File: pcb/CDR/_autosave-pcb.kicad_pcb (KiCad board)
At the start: 2 copper layers, 11 parts, among them J4 Conn_01x03_Male, J5 Conn_01x04_Female, J6 Conn_01x08_Female, J7 Conn_01x02_Female, U1 ATmega328-P, Y1 16MHz

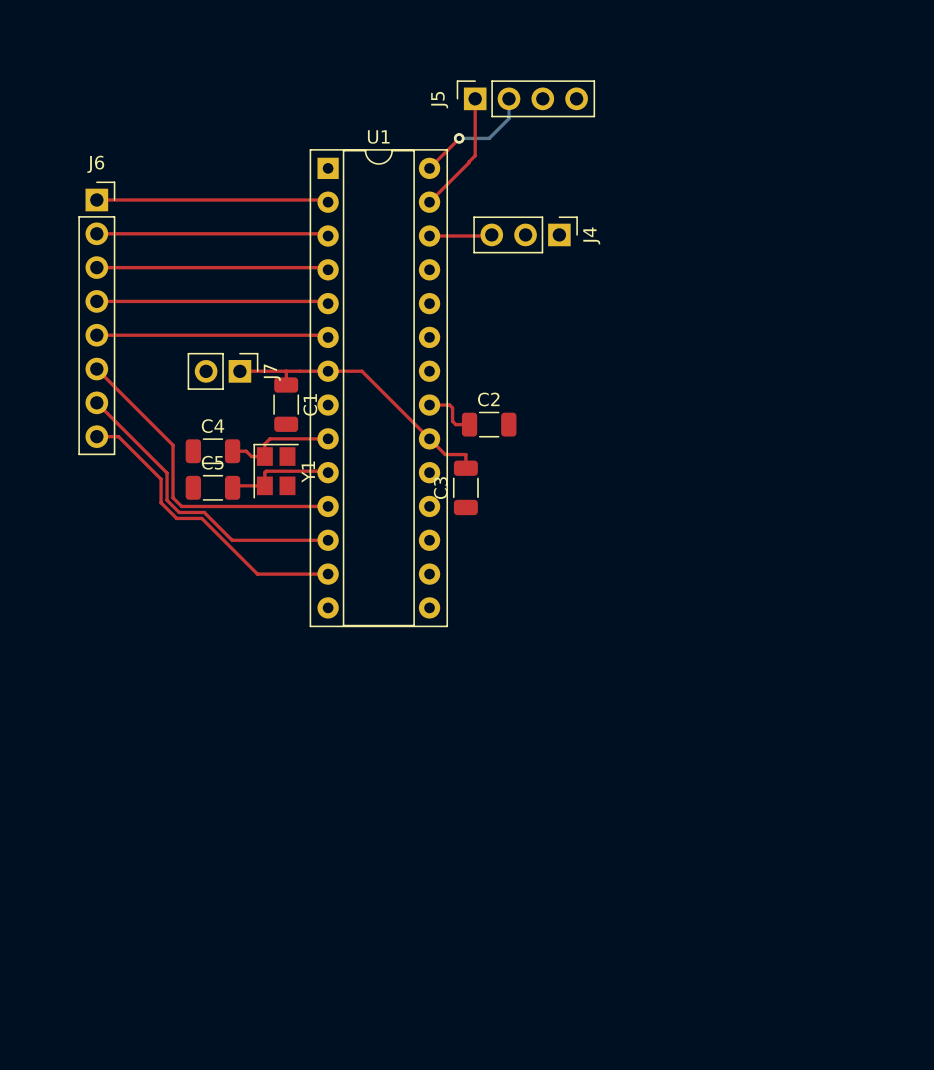
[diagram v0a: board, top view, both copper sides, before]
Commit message: cdr pcb
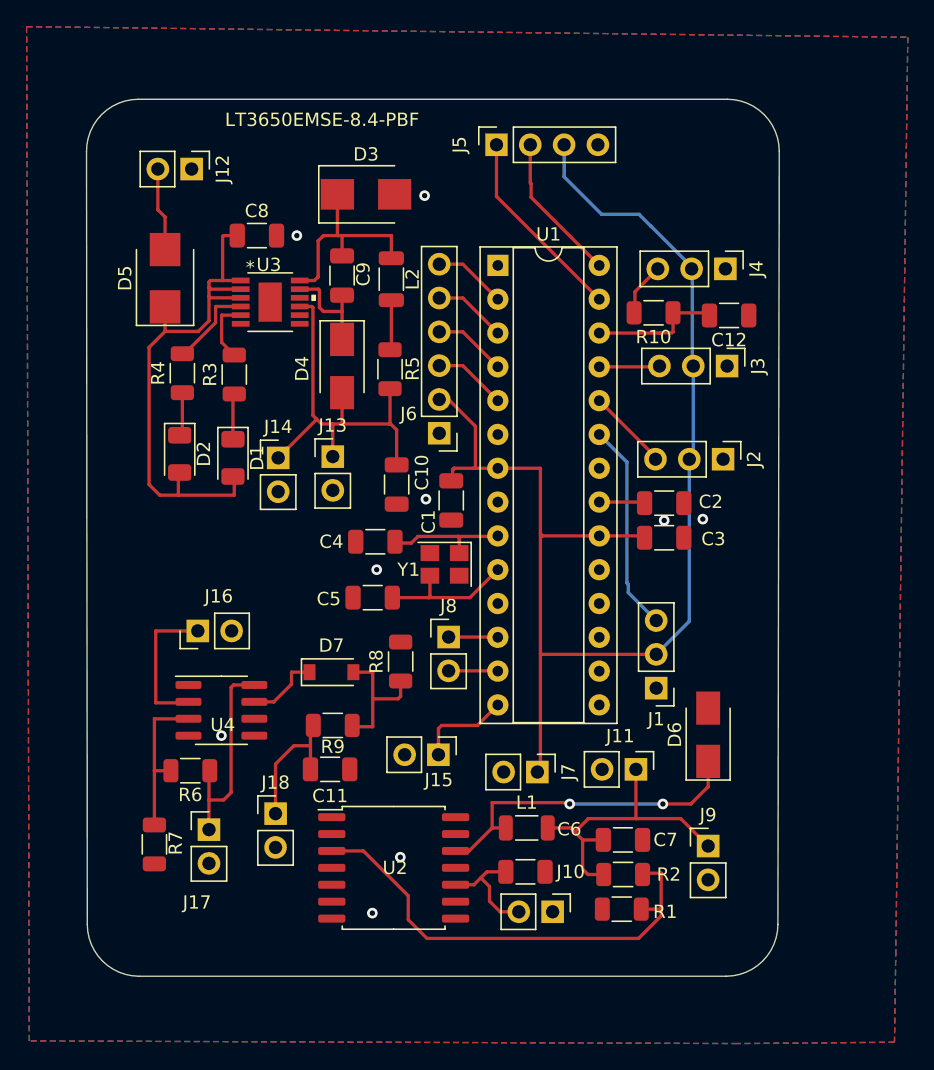
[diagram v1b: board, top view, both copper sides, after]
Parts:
- added C10: 10uF, Capacitor_SMD:C_1206_3216Metric, F.Cu at (128.3, 104.0)
- added C11: 10uF, Capacitor_SMD:C_1206_3216Metric, F.Cu at (123.3, 125.4)
- added C12: 10uF, Capacitor_SMD:C_1206_3216Metric, F.Cu at (153.3, 91.3)
- added C6: 22uF, Capacitor_SMD:C_1206_3216Metric, F.Cu at (138.0, 133.1)
- added C7: 220uF, Capacitor_SMD:C_1206_3216Metric, F.Cu at (145.3, 130.7)
- added C8: 10uF, Capacitor_SMD:C_1206_3216Metric, F.Cu at (117.8, 85.3)
- added C9: 1uF, Capacitor_SMD:C_1206_3216Metric, F.Cu at (124.2, 88.3)
- added D1: Red, Diode_SMD:D_1206_3216Metric, F.Cu at (116.0, 102.0)
- added D2: Green, Diode_SMD:D_1206_3216Metric, F.Cu at (112.0, 101.7)
- added D3: CMPSH3-40MA, Diode_SMD:D_SMB, F.Cu at (126.0, 82.2)
- added D4: CMPSH1-4, Diode_SMD:D_SMA, F.Cu at (124.2, 95.1)
- added D5: CMPSH3-40MA, Diode_SMD:D_SMB, F.Cu at (110.9, 88.5)
- added D6: 11DQ06, Diode_SMD:D_SMA, F.Cu at (151.7, 122.8)
- added D7: 1V, Diode_SMD:D_SOD-123, F.Cu at (123.4, 118.1)
- added J1: Conn_01x03_Male, Connector_PinHeader_2.54mm:PinHeader_1x03_P2.54mm_Vertical, F.Cu at (147.8, 119.3)
- added J10: V Reg in, Connector_PinHeader_2.54mm:PinHeader_1x02_P2.54mm_Vertical, F.Cu at (140.0, 136.1)
- added J11: V reg out, Connector_PinHeader_2.54mm:PinHeader_1x02_P2.54mm_Vertical, F.Cu at (146.3, 125.4)
- added J12: V Solar, Connector_PinHeader_2.54mm:PinHeader_1x02_P2.54mm_Vertical, F.Cu at (112.9, 80.3)
- added J13: V batt, Connector_PinHeader_2.54mm:PinHeader_1x02_P2.54mm_Vertical, F.Cu at (123.5, 101.9)
- added J14: V chrg out, Connector_PinHeader_2.54mm:PinHeader_1x02_P2.54mm_Vertical, F.Cu at (119.4, 102.0)
- added J15: V Low Batt in, Connector_PinHeader_2.54mm:PinHeader_1x02_P2.54mm_Vertical, F.Cu at (131.4, 124.3)
- added J16: V ref in, Connector_PinHeader_2.54mm:PinHeader_1x02_P2.54mm_Vertical, F.Cu at (113.4, 115.0)
- added J17: V Batt in, Connector_PinHeader_2.54mm:PinHeader_1x02_P2.54mm_Vertical, F.Cu at (114.2, 129.9)
- added J18: V Low Batt out, Connector_PinHeader_2.54mm:PinHeader_1x02_P2.54mm_Vertical, F.Cu at (119.2, 128.7)
- added J2: Conn_01x03_Male, Connector_PinHeader_2.54mm:PinHeader_1x03_P2.54mm_Vertical, F.Cu at (152.8, 102.1)
- added J3: Conn_01x03_Male, Connector_PinHeader_2.54mm:PinHeader_1x03_P2.54mm_Vertical, F.Cu at (153.1, 95.1)
- added J8: Cell Module, Connector_PinHeader_2.54mm:PinHeader_1x02_P2.54mm_Vertical, F.Cu at (132.2, 115.5)
- added J9: V reg out, Connector_PinHeader_2.54mm:PinHeader_1x02_P2.54mm_Vertical, F.Cu at (151.7, 131.2)
- added L1: 330 uH, Inductor_SMD:L_1206_3216Metric, F.Cu at (138.1, 129.8)
- added L2: 10uH, Inductor_SMD:L_1206_3216Metric, F.Cu at (127.9, 88.6)
- added R1: 1K, Resistor_SMD:R_1206_3216Metric, F.Cu at (145.2, 135.9)
- added R10: 0/160, Resistor_SMD:R_1206_3216Metric, F.Cu at (147.6, 91.1)
- added R2: 3.1k, Resistor_SMD:R_1206_3216Metric, F.Cu at (145.3, 133.3)
- added R3: 5.1k, Resistor_SMD:R_1206_3216Metric, F.Cu at (116.1, 95.7)
- added R4: 5.1k, Resistor_SMD:R_1206_3216Metric, F.Cu at (112.2, 95.6)
- added R5: 0.05, Resistor_SMD:R_1206_3216Metric, F.Cu at (127.8, 95.3)
- added R6: 100k, Resistor_SMD:R_1206_3216Metric, F.Cu at (112.8, 125.5)
- added R7: 220k, Resistor_SMD:R_1206_3216Metric, F.Cu at (110.1, 131.0)
- added R8: 50k, Resistor_SMD:R_1206_3216Metric, F.Cu at (128.6, 117.3)
- added R9: 160, Resistor_SMD:R_1206_3216Metric, F.Cu at (123.5, 122.1)
- added U2: LM2574HVM-12, Package_SO:SOIC-14W_7.5x9mm_P1.27mm, F.Cu at (128.1, 132.8)
- added U3: LT3650EMSE-8.4-PBF, footprints:LT3650EMSE-8.4-PBF, F.Cu at (118.8, 90.3)
- added U4: LM311, Package_SO:SOIC-8_3.9x4.9mm_P1.27mm, F.Cu at (115.1, 121.0)
- J6: value Conn_01x08_Female -> SD Card Reader; footprint Connector_PinSocket_2.54mm:PinSocket_1x08_P2.54mm_Vertical -> Connector_PinHeader_2.54mm:PinHeader_1x06_P2.54mm_Vertical
- J7: value Conn_01x02_Female -> V sys in
- Y1: footprint Crystal:Crystal_SMD_3225-4Pin_3.2x2.5mm -> Crystal:Crystal_SMD_TXC_7M-4Pin_3.2x2.5mm
- moved J7 37.5 mm to (138.9, 125.6)
- moved J6 31.1 mm to (131.5, 100.2), turned to 180 degrees
- moved C3 15.4 mm to (148.4, 108.0), turned to 180 degrees
- moved U1 14.7 mm to (135.9, 87.5)
- moved C5 14.6 mm to (126.5, 112.5)
- moved Y1 14.5 mm to (131.9, 110.0), turned to 180 degrees
- moved C2 14.4 mm to (148.4, 105.4)
- moved C1 14.3 mm to (132.4, 105.2)
- moved C4 14.0 mm to (126.7, 108.3)
- moved J4 12.7 mm to (153.0, 87.8)
- moved J5 3.80 mm to (135.8, 78.5)
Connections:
- J6 pad 1: Net-(J6-Pad1) -> GND
- J6 pad 2: Net-(J6-Pad2) -> VCC
- U1 pad 11: Net-(J6-Pad6) -> unconnected-(U1-Pad11)
- U1 pad 12: Net-(J6-Pad7) -> Net-(J8-Pad1)
- U1 pad 13: Net-(J6-Pad8) -> Net-(J8-Pad2)
- U1 pad 14: unconnected-(U1-Pad14) -> Net-(J15-Pad1)
- U1 pad 2: Net-(J6-Pad1) -> Net-(J6-Pad6)
- U1 pad 26: Net-(J4-Pad3) -> Net-(C12-Pad2)
- U1 pad 3: Net-(J6-Pad2) -> Net-(J6-Pad5)
- U1 pad 4: Net-(J6-Pad3) -> Net-(J6-Pad4)
- U1 pad 5: Net-(J6-Pad4) -> Net-(J6-Pad3)
- U1 pad 6: Net-(J6-Pad5) -> unconnected-(U1-Pad6)
- Y1 pad 2: Net-(C5-Pad2) -> GND
- Y1 pad 3: (no net) -> Net-(C5-Pad2)
- Y1 pad 4: (no net) -> GND
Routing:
- net VCC: track 21.7 -> 98.5 mm
- net Net-(C8-Pad1): track 0.00 -> 42.0 mm
- net Net-(R1-Pad2): track 0.00 -> 35.6 mm
- net Net-(C10-Pad1): track 0.00 -> 30.1 mm
- net Net-(D6-Pad1): track 0.00 -> 25.1 mm, vias 0 -> 2
- net Net-(C7-Pad1): track 0.00 -> 23.5 mm
- net Net-(J6-Pad7): track 22.9 -> 0.00 mm
- net Net-(J6-Pad8): track 22.7 -> 0.00 mm
- net Net-(J6-Pad6): track 24.0 -> 4.79 mm
- net Net-(J6-Pad1): track 17.4 -> 0.00 mm
- net Net-(J6-Pad2): track 17.4 -> 0.00 mm
- net Net-(C9-Pad1): track 0.00 -> 16.2 mm
- net Net-(J17-Pad1): track 0.00 -> 16.1 mm
- net Net-(J1-Pad3): track 0.00 -> 15.8 mm
- net Net-(J6-Pad5): track 17.4 -> 4.79 mm
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- added copper zone on B.Cu, net GND
- added copper zone on F.Cu, net GND
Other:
- board outline added: 52 x 65.9 mm
